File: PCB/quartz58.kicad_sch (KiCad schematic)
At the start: 188 parts, among them J1 OLED_128x32, J2 OLED_128x32, SW1 SW_SPDT, SW2 SW_Push_Shielded, SW4 SW_SPDT, SW5 SW_Push_Shielded, T1 TPS65-201A-S, U1 Nice_Nano_V2, U4 Nice_Nano_V2

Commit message: more progress?
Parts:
- BT1, BT2: footprint (none) -> ScottoKeebs_Components:Connector_1x02_JST-PH
- D1, D10, D11, D12, D13, D14, D15, D16, D17, D18, D19, D2, D20, D21, D22, D23, D24, D25, D26, D27, D28, D29, D3, D4, D5, D6, D64, D65, D66, D67, D68, D69, D7, D70, D71, D72, D73, D74, D75, D76, D77, D78, D79, D8, D80, D81, D82, D83, D84, D85, D86, D87, D88, D89, D9, D90, D91, D92: footprint (none) -> ScottoKeebs_Components:Diode_SOD-123
- D100, D101, D102, D103, D104, D105, D106, D107, D108, D109, D110, D111, D112, D113, D114, D115, D116, D117, D118, D119, D120, D121, D30, D31, D32, D33, D34, D35, D36, D37, D38, D39, D40, D41, D42, D43, D44, D45, D46, D47, D48, D49, D50, D51, D52, D53, D54, D55, D56, D57, D58, D93, D94, D95, D96, D97, D98, D99: footprint ScottoKeebs_Components:LED_SK6812MINI -> Keebio-Parts.pretty-master:SK6812-MINI-E
- S1, S10, S11, S12, S13, S14, S15, S16, S17, S18, S19, S2, S20, S21, S22, S23, S24, S25, S26, S27, S28, S29, S3, S35, S36, S37, S38, S39, S4, S40, S41, S42, S43, S44, S45, S46, S47, S48, S49, S5, S50, S51, S52, S53, S54, S55, S56, S57, S58, S59, S6, S60, S61, S62, S63, S7, S8, S9: footprint (none) -> Hotswap_Choc_and_MX:Hotswap_Choc_V1V2
- U1, U4: footprint ScottoKeebs_MCU:Nice_Nano_V2 -> nice-nano-kicad-master:nice_nano

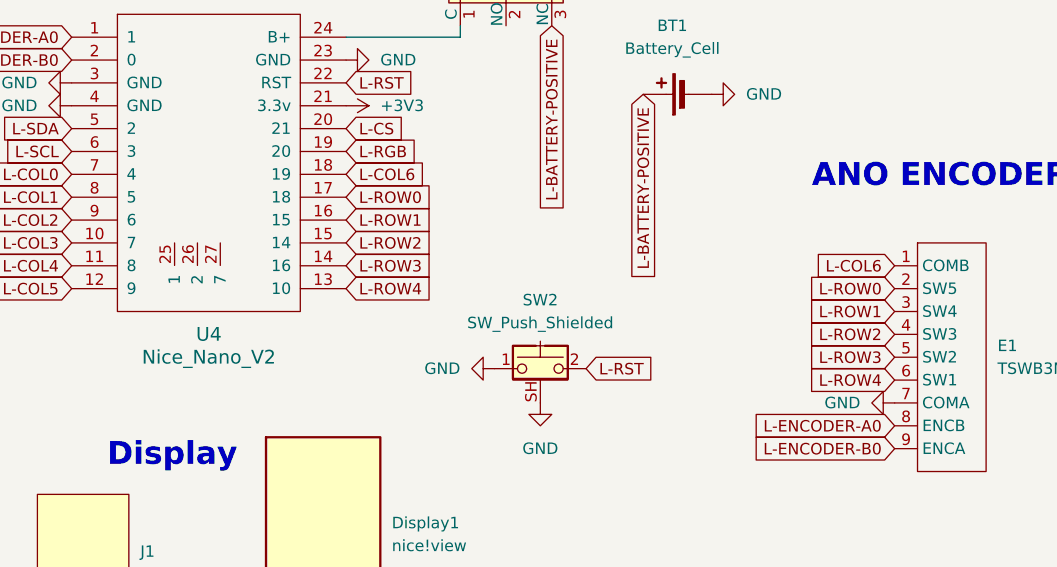
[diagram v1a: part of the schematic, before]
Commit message: coming back
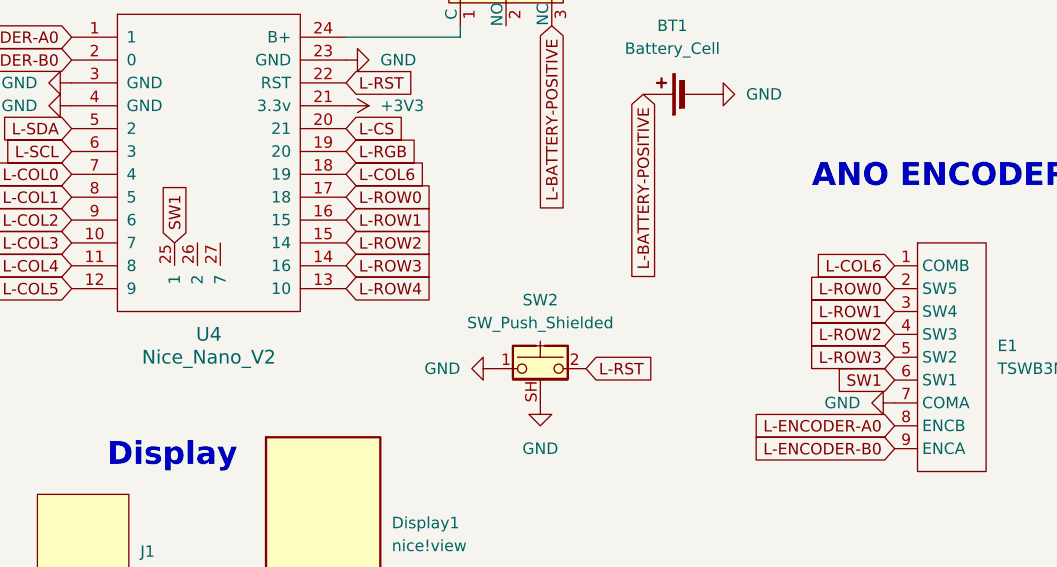
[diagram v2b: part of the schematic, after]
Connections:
- net L-ROW4: no longer E1.6 (SW1)
- net SW1: now reaches U4.25 (1)
- net SW1: now also E1.6 (SW1)
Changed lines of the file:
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@@
+		)
+	)
+	(global_label "SW1"
+		(shape input)
+		(at 45.72 187.96 90)
+		(fields_autoplaced yes)
+		(effects
+			(font
+				(size 1.27 1.27)
+			)
+			(justify left)
+		)
+		(property "Intersheetrefs" "${INTERSHEET_REFS}"
+			(at 45.72 181.1044 90)
+			(effects
+				(font
+					(size 1.27 1.27)
+				)
+				(justify left)
+				(hide yes)
+			)
 		)
 	)
@@
 		)
 	)
+	(global_label "SW1"
+		(shape input)
+		(at 125.73 203.2 180)
+		(fields_autoplaced yes)
+		(effects
+			(font
+				(size 1.27 1.27)
+			)
+			(justify right)
+		)
+		(property "Intersheetrefs" "${INTERSHEET_REFS}"
+			(at 118.8744 203.2 0)
+			(effects
+				(font
+					(size 1.27 1.27)
+				)
+				(justify right)
+				(hide yes)
+			)
+		)
+	)
 	(global_label "R-RGB"
 		(shape input)
@@
 			(effects
 				(font
-					(size 1.27 1.27)
-				)
-				(justify right)
-				(hide yes)
-			)
-		)
-	)
-	(global_label "L-ROW4"
-		(shape input)
-		(at 125.73 203.2 180)
-		(fields_autoplaced yes)
-		(effects
-			(font
-				(size 1.27 1.27)
-			)
-			(justify right)
-		)
-		(property "Intersheetrefs" "${INTERSHEET_REFS}"
-			(at 114.8829 203.2 0)
-			(effects
-				(font

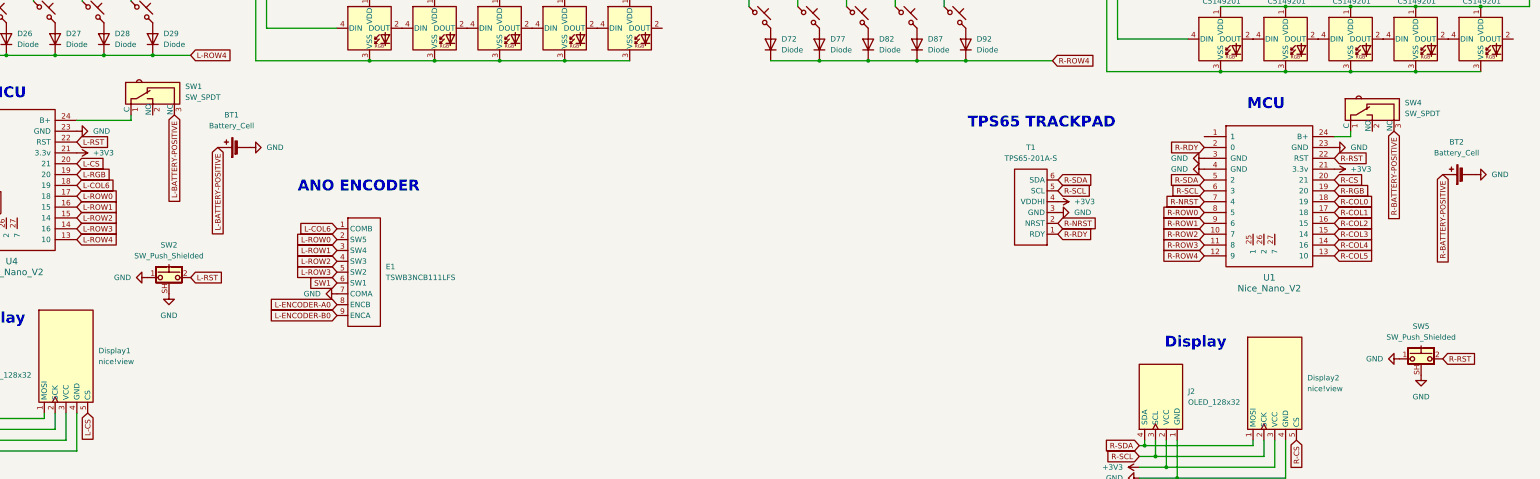
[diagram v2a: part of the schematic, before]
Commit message: pcb and cad updates
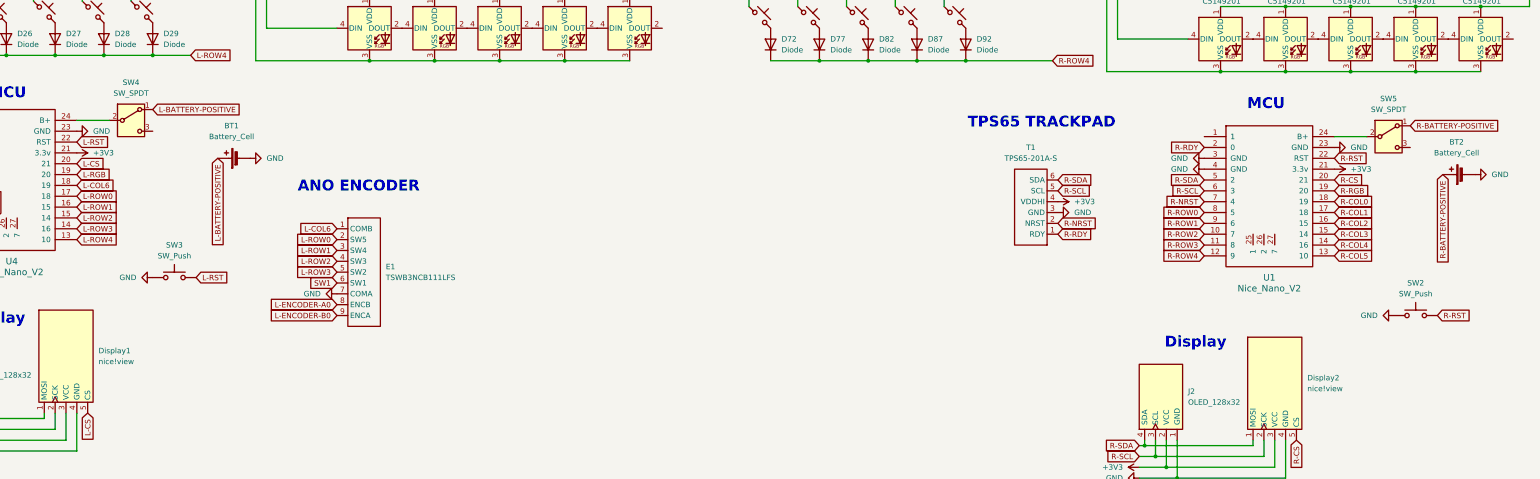
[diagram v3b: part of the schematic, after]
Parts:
- removed SW1, SW4: SW_SPDT, openinput:SW_Micro_Switch, symbol PCM_openinput:SW_SPDT
- removed SW2, SW5: SW_Push_Shielded, symbol Switch:SW_Push_Shielded
- added SW2, SW3: SW_Push, ul_EVQ-PUJ02K:SW_EVQPUJ_4P7X3P5_PAN, symbol Switch:SW_Push
- added SW4, SW5: SW_SPDT, SSSS811101:SW_SSSS811101, symbol Switch:SW_SPDT
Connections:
- net GND: now also SW2.1, SW3.1
- net L-BATTERY-POSITIVE: now also SW4.1 (A)
- net L-RST: now also SW3.2
- net R-BATTERY-POSITIVE: now also SW5.1 (A)
- net R-RST: now also SW2.2
- net at U4.24 (B+): now also SW4.2 (B)
- net at U1.24 (B+): now also SW5.2 (B)
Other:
- moved on the sheet: BT1
